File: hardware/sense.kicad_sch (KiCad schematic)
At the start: 9 parts, among them U10 AS5048A

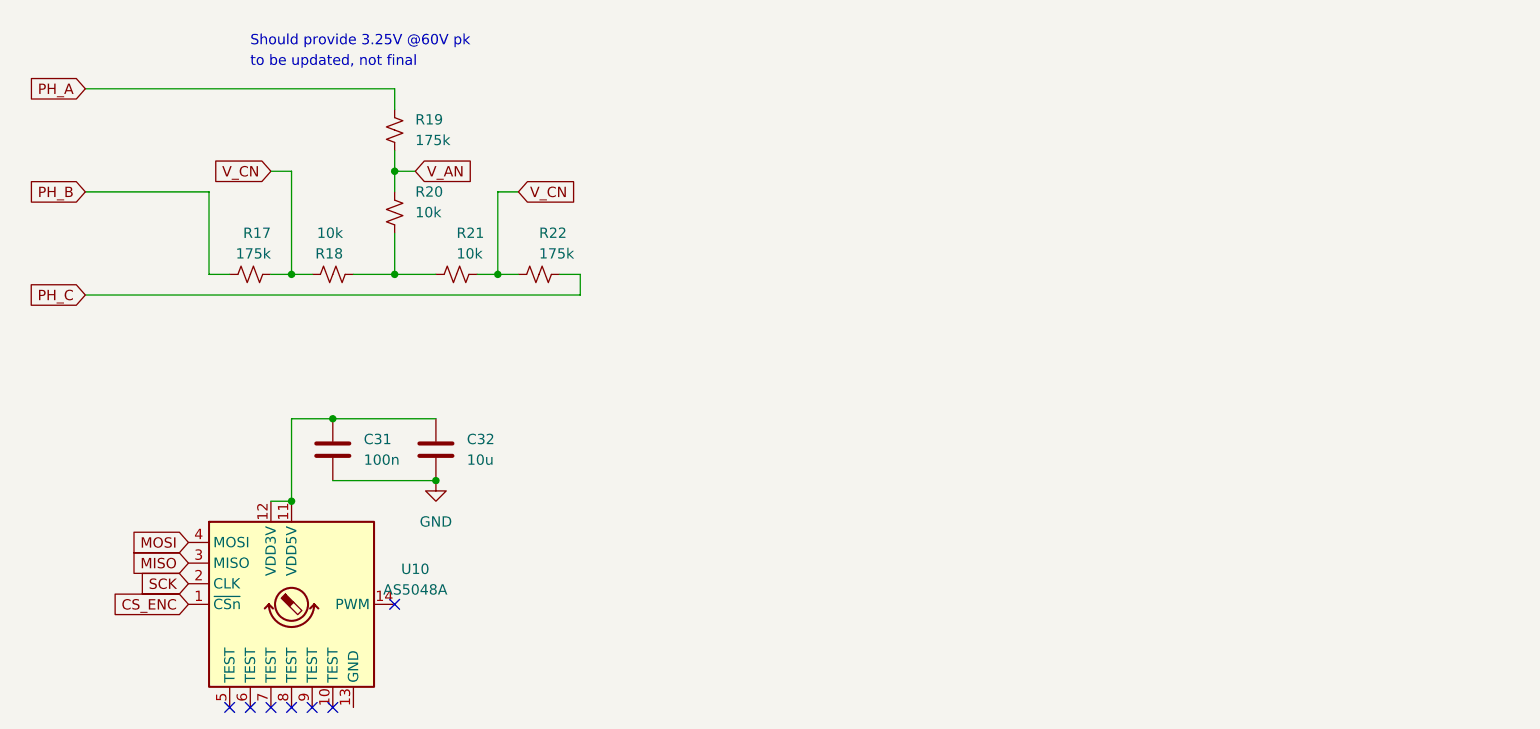
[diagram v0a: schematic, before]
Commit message: Net changes, sense changes
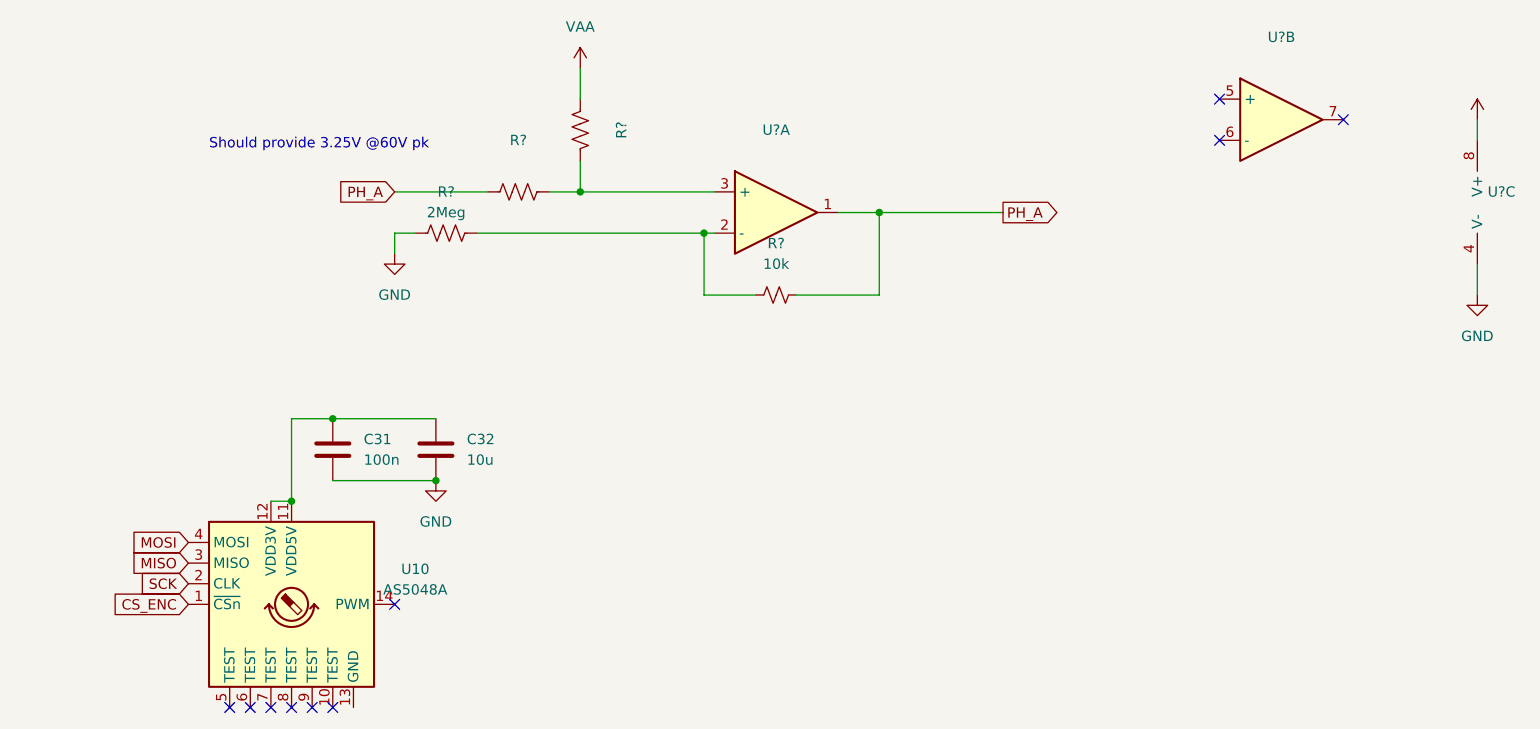
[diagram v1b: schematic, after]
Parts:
- removed R17, R19, R22: 175k, symbol Device:R_Small_US
- removed R18, R20, R21: 10k, symbol Device:R_Small_US
- added R? (x2): (no value), Resistor_SMD:R_0805_2012Metric, symbol Device:R_US
- added R?: 2Meg, Resistor_SMD:R_0805_2012Metric, symbol Device:R_US
- added R?: 10k, Resistor_SMD:R_0805_2012Metric, symbol Device:R_Small_US
- added U? (x3): (no value), symbol Device:Opamp_Dual
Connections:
- net GND: now also R?.1, U?.4 (V-)
- net PH_A: now also R?.1, R?.2, U?.1
- new net: R?.1, R?.2, U?.3 (+)
- new net: R?.1, R?.2, U?.2 (-)
- new net +12V: U?.8 (V+)
- new net VAA: R?.2
- no-connect marks 7 -> 10
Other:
- note removed: "to be updated, not final"
